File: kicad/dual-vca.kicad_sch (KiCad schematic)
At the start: 63 parts, among them J1 Eurorack Mono Jack, J11 Conn_01x06_Socket, J12 Conn_01x06_Pin, J2 Eurorack Mono Jack, J3 Eurorack Mono Jack, J4 Eurorack Mono Jack, J5 Eurorack Power Small, J6 Eurorack Mono Jack, J7 Eurorack Mono Jack, J8 Conn_01x06_Pin, J9 Conn_01x06_Socket, U1 SSI2164, U2 TL074, U3 LM4040LP-10, U4 LM4040LP-2.5

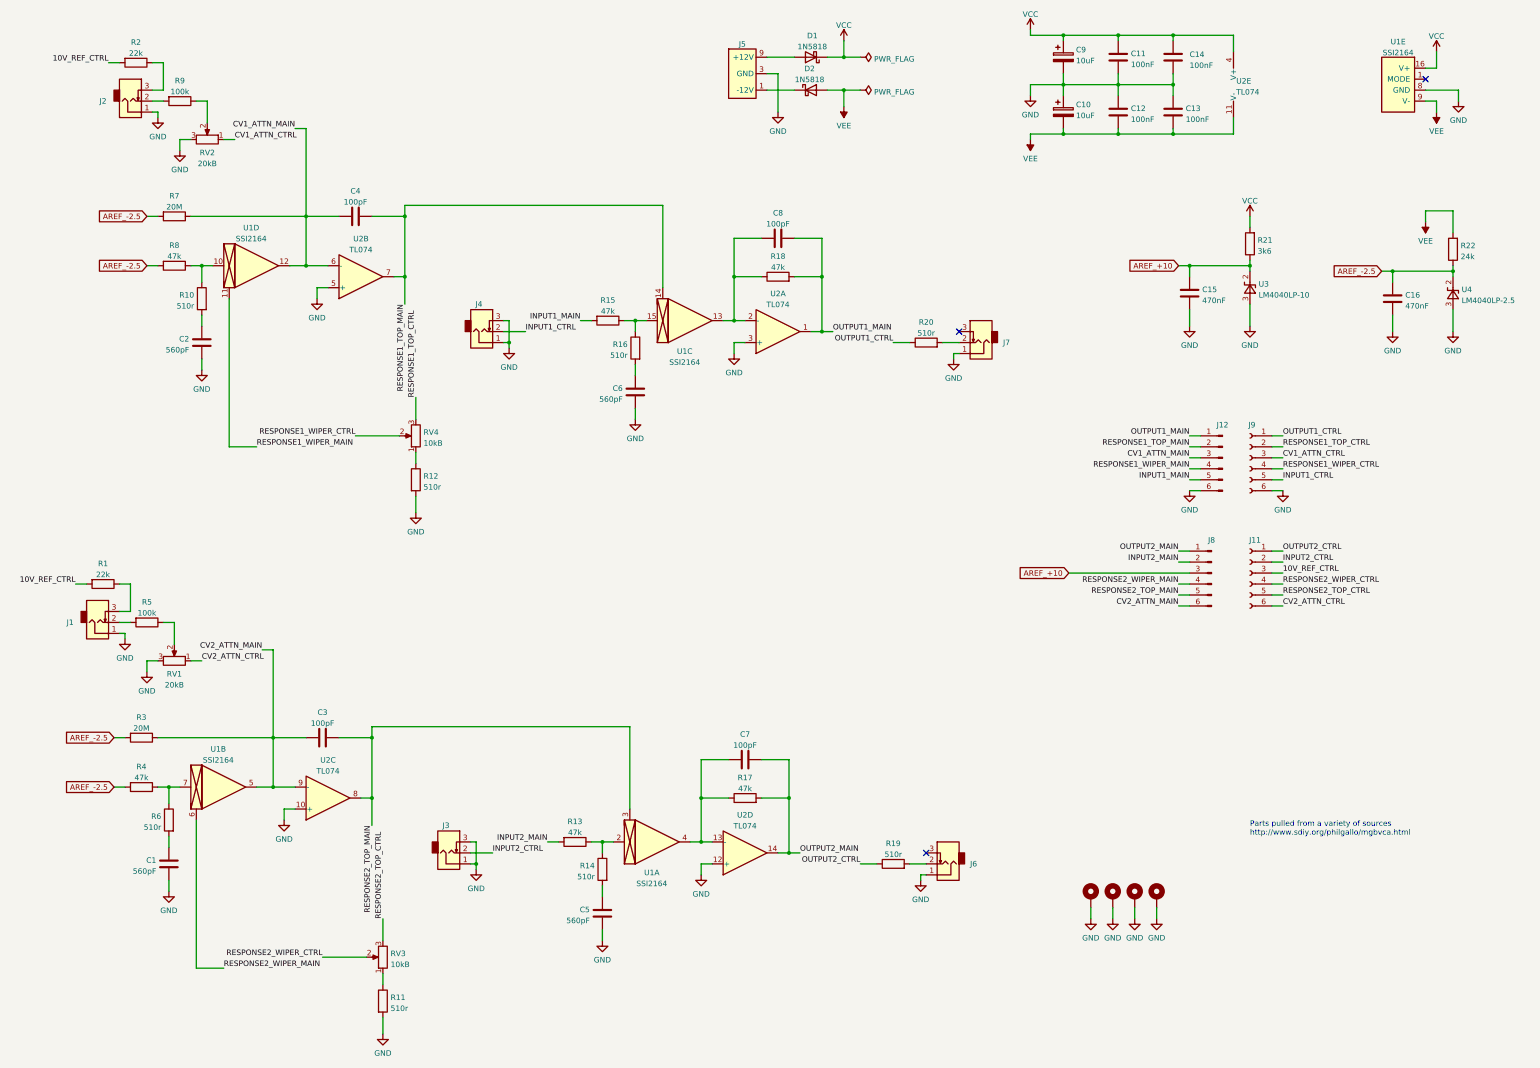
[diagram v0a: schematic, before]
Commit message: Finishing routing PCBs
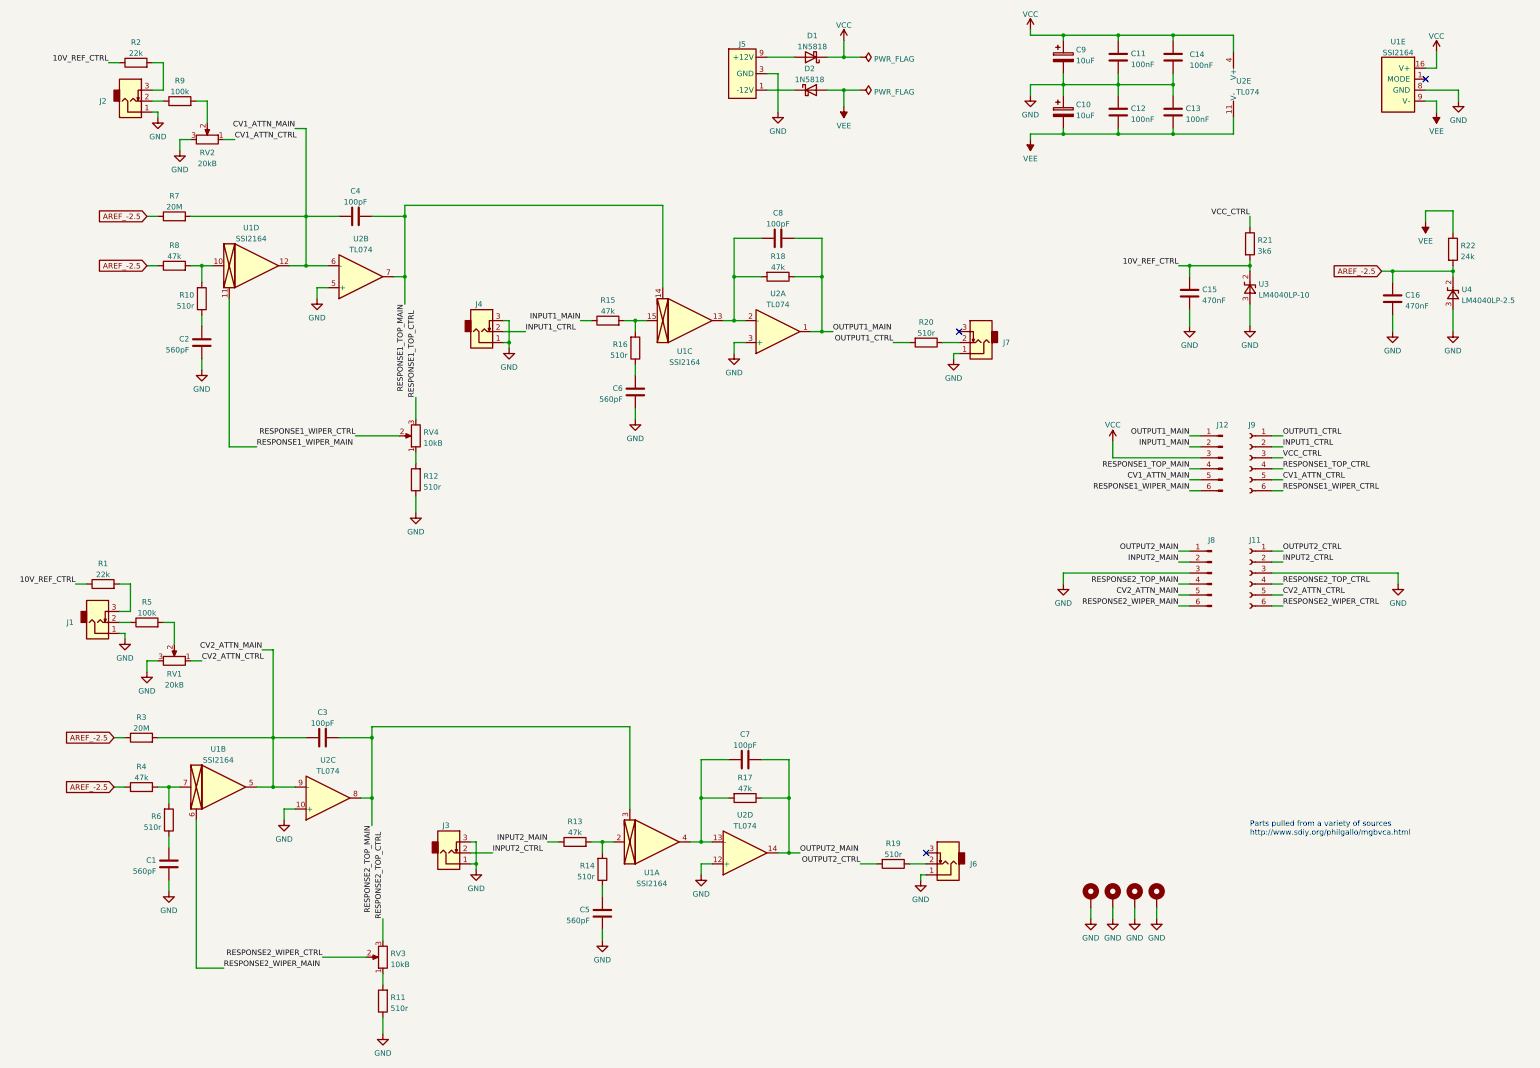
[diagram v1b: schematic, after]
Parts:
- C1, C11, C12, C13, C14, C15, C16, C2, C3, C4, C5, C6, C7, C8: footprint Rumblesan_Standard_Parts:C_Rect_L7.0mm_W2.5mm_P5.00mm -> Capacitor_THT:C_Rect_L7.0mm_W2.5mm_P5.00mm; symbol rumblesan-standard-parts:C -> Device:C
- C10, C9: footprint Rumblesan_Standard_Parts:CP_Radial_D5.0mm_P2.00mm -> Capacitor_THT:CP_Radial_D5.0mm_P2.00mm; symbol rumblesan-standard-parts:C_Polarized -> Device:C_Polarized
- D1, D2: footprint Rumblesan_Standard_Parts:D_DO-41_SOD81_P10.16mm_Horizontal -> Diode_THT:D_DO-41_SOD81_P10.16mm_Horizontal
- J5: symbol Eurorack_Hardware:Eurorack Power Small -> Eurorack_Power:Eurorack Power Small
- R1, R10, R11, R12, R13, R14, R15, R16, R17, R18, R19, R2, R20, R21, R22, R3, R4, R5, R6, R7, R8, R9: footprint Rumblesan_Standard_Parts:R_Axial_DIN0207_L6.3mm_D2.5mm_P10.16mm_Horizontal -> Resistor_THT:R_Axial_DIN0207_L6.3mm_D2.5mm_P10.16mm_Horizontal; symbol rumblesan-standard-parts:R -> Device:R
- U3, U4: footprint Package_TO_SOT_THT:TO-92_Inline -> Package_TO_SOT_THT:TO-92_Inline_Wide
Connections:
- net 10V_REF_CTRL: now also C15.1, R1.1, R2.1, R21.2, U3.2 (K); no longer J11.3 (Pin_3), R1.2, R2.2
- net AREF_-2.5: now also R22.2, R3.1, R4.1, R7.1, R8.1; no longer R22.1, R3.2, R4.2, R7.2, R8.2
- net CV1_ATTN_CTRL: now also J9.5 (Pin_5); no longer J9.3 (Pin_3)
- net CV1_ATTN_MAIN: now also J12.5 (Pin_5), R7.2; no longer J12.3 (Pin_3), R7.1
- net CV2_ATTN_CTRL: now also J11.5 (Pin_5); no longer J11.6 (Pin_6)
- net CV2_ATTN_MAIN: now also J8.5 (Pin_5), R3.2; no longer J8.6 (Pin_6), R3.1
- net GND: now also J11.3 (Pin_3), J8.3 (Pin_3), R11.1, R12.1; no longer J12.6 (Pin_6), J9.6 (Pin_6), R11.2, R12.2
- net INPUT1_CTRL: now also J9.2 (Pin_2); no longer J9.5 (Pin_5)
- net INPUT1_MAIN: now also J12.2 (Pin_2), R15.1; no longer J12.5 (Pin_5), R15.2
- net INPUT2_MAIN: now also R13.1; no longer R13.2
- net OUTPUT1_CTRL: now also R20.2; no longer R20.1
- net OUTPUT1_MAIN: now also R18.1; no longer R18.2
- net OUTPUT2_CTRL: now also R19.2; no longer R19.1
- net OUTPUT2_MAIN: now also R17.1; no longer R17.2
- net RESPONSE1_TOP_CTRL: now also J9.4 (Pin_4); no longer J9.2 (Pin_2)
- net RESPONSE1_TOP_MAIN: now also J12.4 (Pin_4); no longer J12.2 (Pin_2)
- net RESPONSE1_WIPER_CTRL: now also J9.6 (Pin_6); no longer J9.4 (Pin_4)
- net RESPONSE1_WIPER_MAIN: now also J12.6 (Pin_6); no longer J12.4 (Pin_4)
- net RESPONSE2_TOP_CTRL: now also J11.4 (Pin_4); no longer J11.5 (Pin_5)
- net RESPONSE2_TOP_MAIN: now also J8.4 (Pin_4); no longer J8.5 (Pin_5)
- net RESPONSE2_WIPER_CTRL: now also J11.6 (Pin_6); no longer J11.4 (Pin_4)
- net RESPONSE2_WIPER_MAIN: now also J8.6 (Pin_6); no longer J8.4 (Pin_4)
- net VCC: now also J12.3 (Pin_3); no longer R21.2
- net VEE: now also R22.1; no longer R22.2
- net at C8.1, U1.13, U2.2 (-): now also R18.2; no longer R18.1
- net at RV4.1: now also R12.2; no longer R12.1
- net at J2.3 (Tip_normalize): now also R2.2; no longer R2.1
- net at RV3.1: now also R11.2; no longer R11.1
- net at C7.1, U1.4, U2.13 (-): now also R17.2; no longer R17.1
- net at J6.2 (Tip): now also R19.1; no longer R19.2
- net at J1.2 (Tip): now also R5.1; no longer R5.2
- net at J1.3 (Tip_normalize): now also R1.2; no longer R1.1
- net at RV1.2: now also R5.2; no longer R5.1
- net at C5.2: now also R14.1; no longer R14.2
- net at R16.2: now also R15.2, U1.15; no longer C6.2
- net at C1.2: now also R6.1; no longer R6.2
- net at R9.1: now also J2.2 (Tip); no longer RV2.2
- net at R9.2: now also RV2.2; no longer J2.2 (Tip)
- net at R10.2: now also R8.2, U1.10; no longer C2.2
- net at J7.2 (Tip): now also R20.1; no longer R20.2
- removed net AREF_+10: C15.1, J8.3 (Pin_3), R21.1, U3.2 (K)
- new net: C6.2, R16.1
- new net: R4.2, R6.2, U1.7
- new net: R13.2, R14.2, U1.2
- new net: C2.2, R10.1
- new net VCC_CTRL: J9.3 (Pin_3), R21.1
